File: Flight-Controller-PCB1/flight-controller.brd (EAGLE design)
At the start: 100 x 25.4 mm, 37 parts, among them J1 1981584-1, U1 MK20DX256VLH7, U2 TPS61200, U3 MINI54TAN, Y1 32.768KHz, Y2 16Mhz/8pF

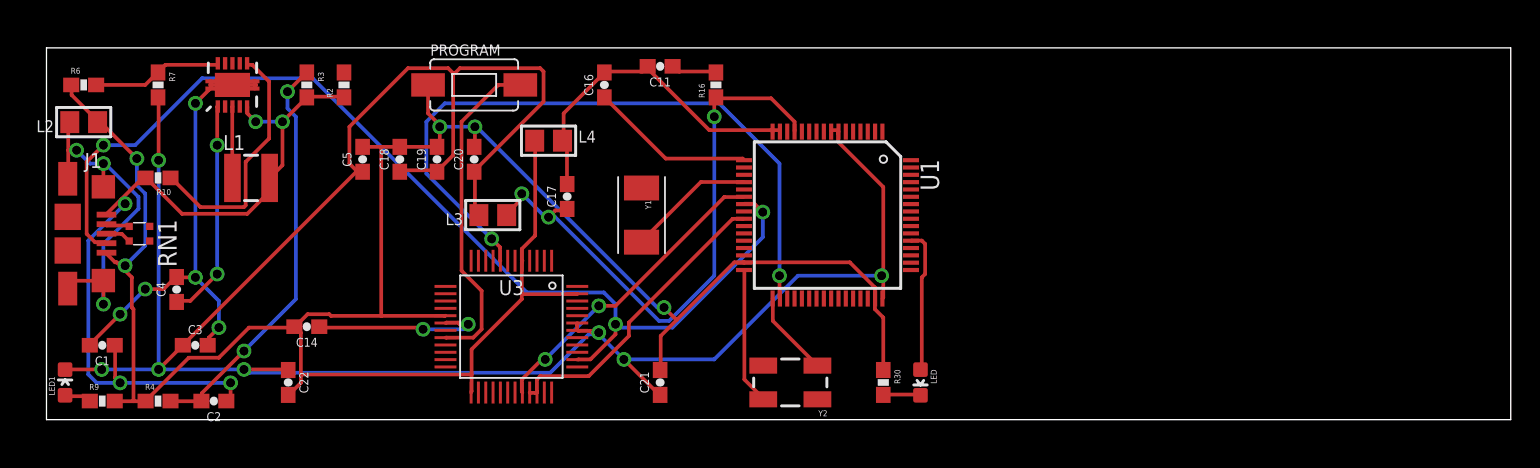
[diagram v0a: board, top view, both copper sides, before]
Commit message: update
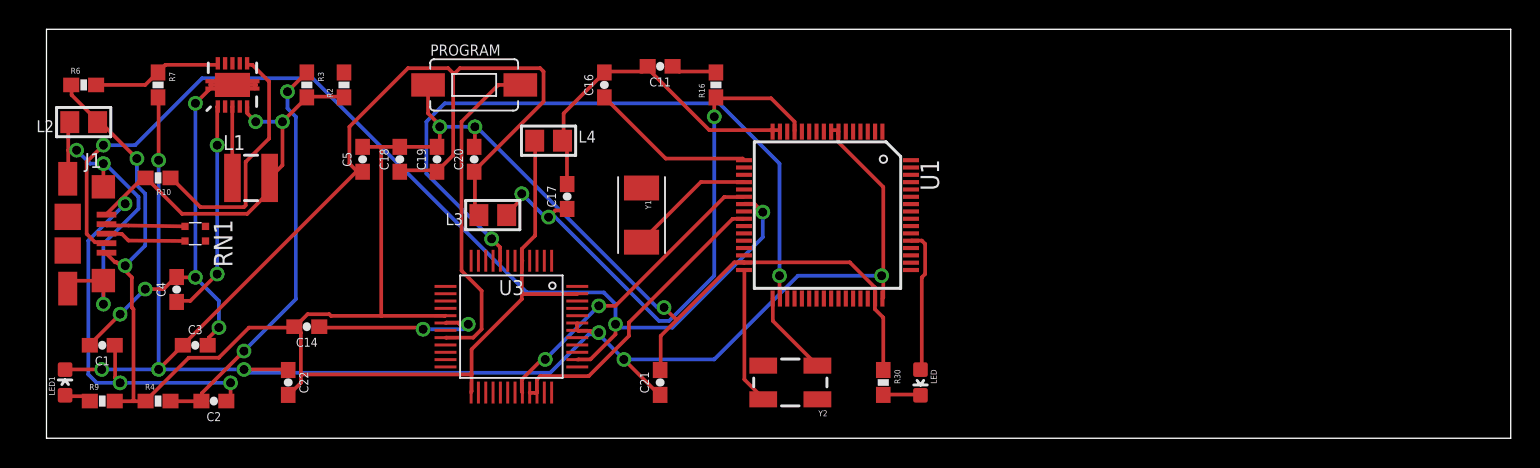
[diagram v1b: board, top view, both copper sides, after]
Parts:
- moved RN1 3.81 mm to (10.2, 12.7)
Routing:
- net USB_CON_P: track 1.75 -> 5.55 mm
- net USB_CON_N: track 1.66 -> 5.44 mm
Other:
- board size 100 x 25.4 mm -> 100 x 27.9 mm
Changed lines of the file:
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@@
 <board>
 <plain>
-<wire x1="0" y1="0" x2="100" y2="0" width="0" layer="20"/>
-<wire x1="100" y1="0" x2="100" y2="25.39" width="0" layer="20"/>
-<wire x1="100" y1="25.39" x2="0" y2="25.39" width="0" layer="20"/>
-<wire x1="0" y1="25.39" x2="0" y2="0" width="0" layer="20"/>
+<wire x1="0" y1="-1.27" x2="100" y2="-1.27" width="0" layer="20"/>
+<wire x1="100" y1="-1.27" x2="100" y2="26.66" width="0" layer="20"/>
+<wire x1="100" y1="26.66" x2="0" y2="26.66" width="0" layer="20"/>
+<wire x1="0" y1="26.66" x2="0" y2="-1.27" width="0" layer="20"/>
 </plain>
 <attributes>
@@
 <attribute name="MF" value="Panasonic" x="3.81" y="1.27" size="1.778" layer="27" display="off"/>
 </element>
-<element name="RN1" library="resistor-dil" package="EXB34V" value="33" x="6.35" y="12.7" rot="R270">
-<attribute name="MPN" value="EXB-34V330JV" x="6.35" y="12.7" size="1.778" layer="27" rot="R270" display="off"/>
-<attribute name="OC_NEWARK" value="unknown" x="6.35" y="12.7" size="1.778" layer="27" rot="R270" display="off"/>
-<attribute name="MF" value="Panasonic" x="6.35" y="12.7" size="1.778" layer="27" rot="R270" display="off"/>
-<attribute name="OC_FARNELL" value="unknown" x="6.35" y="12.7" size="1.778" layer="27" rot="R270" display="off"/>
+<element name="RN1" library="resistor-dil" package="EXB34V" value="33" x="10.16" y="12.7" rot="R270">
+<attribute name="MPN" value="EXB-34V330JV" x="10.16" y="12.7" size="1.778" layer="27" rot="R270" display="off"/>
+<attribute name="OC_NEWARK" value="unknown" x="10.16" y="12.7" size="1.778" layer="27" rot="R270" display="off"/>
+<attribute name="MF" value="Panasonic" x="10.16" y="12.7" size="1.778" layer="27" rot="R270" display="off"/>
+<attribute name="OC_FARNELL" value="unknown" x="10.16" y="12.7" size="1.778" layer="27" rot="R270" display="off"/>
 </element>
 <element name="U1" library="appfruits" package="MK20DX256VLH7" value="MK20DX256VLH7" x="53.34" y="13.97" rot="R270">
@@
 <contactref element="U1" pad="5"/>
 <contactref element="RN1" pad="3"/>
-<wire x1="7.05" y1="12.2" x2="55.09" y2="19.67" width="0" layer="19" extent="1-1"/>
+<wire x1="10.86" y1="12.2" x2="55.09" y2="19.67" width="0" layer="19" extent="1-1"/>
 </signal>
 <signal name="USB_D_N" class="1">
 <contactref element="RN1" pad="4"/>
 <contactref element="U1" pad="6"/>
-<wire x1="7.05" y1="13.2" x2="54.59" y2="19.67" width="0" layer="19" extent="1-1"/>
+<wire x1="10.86" y1="13.2" x2="54.59" y2="19.67" width="0" layer="19" extent="1-1"/>
 </signal>
 <signal name="ID">
@@
 <contactref element="RN1" pad="1"/>
 <wire x1="4.1148" y1="13.2588" x2="5.6007" y2="13.2588" width="0.254" layer="1"/>
-<wire x1="5.6007" y1="13.2588" x2="5.65" y2="13.2" width="0.254" layer="1"/>
+<wire x1="5.6007" y1="13.2588" x2="9.46" y2="13.2" width="0.254" layer="1"/>
 <wire x1="4.1148" y1="13.2588" x2="4.1" y2="13.35" width="0.254" layer="1"/>
 </signal>
@@
 <wire x1="5.1435" y1="12.6873" x2="5.6007" y2="12.2301" width="0.254" layer="1"/>
 <wire x1="4.1148" y1="12.6873" x2="5.1435" y2="12.6873" width="0.254" layer="1"/>
-<wire x1="5.6007" y1="12.2301" x2="5.65" y2="12.2" width="0.254" layer="1"/>
+<wire x1="5.6007" y1="12.2301" x2="9.46" y2="12.2" width="0.254" layer="1"/>
 <wire x1="4.1148" y1="12.6873" x2="4.1" y2="12.7" width="0.254" layer="1"/>
 </signal>

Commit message: started manually routing
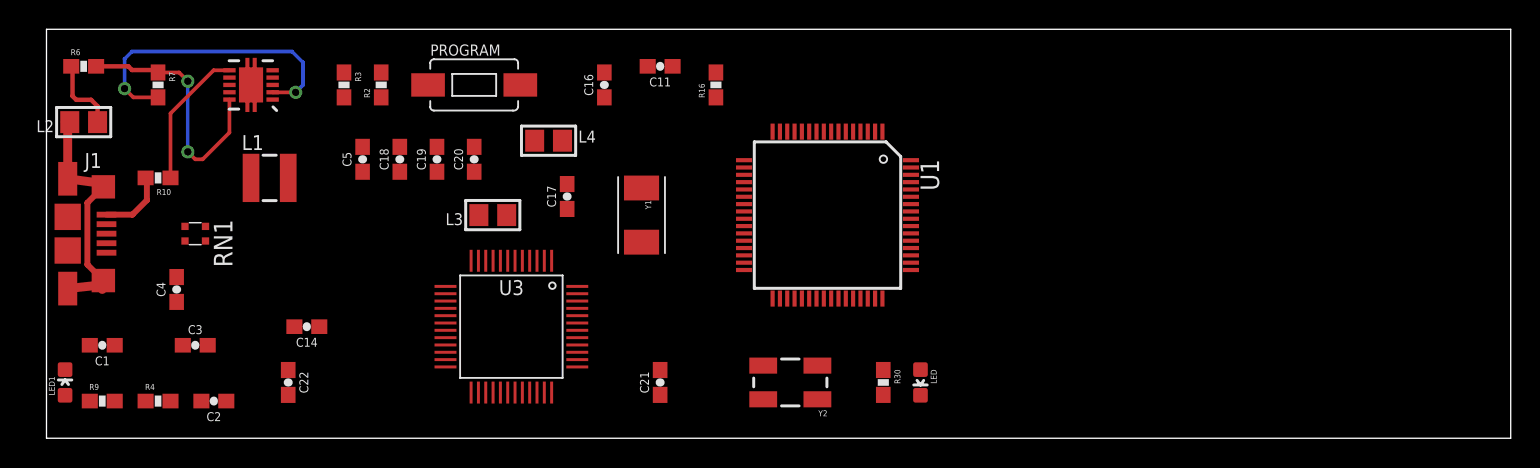
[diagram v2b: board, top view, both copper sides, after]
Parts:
- moved R2 2.54 mm to (22.9, 22.9)
- moved R3 2.54 mm to (20.3, 22.9)
- moved U2 1.27 mm to (14.0, 22.9), turned to 90 degrees
- moved L1 1.27 mm to (15.2, 16.5)
- moved R6 1.27 mm to (2.54, 24.1)
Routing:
- net GND: track 161.3 -> 5.15 mm, vias 5 -> 0
- net 3.3V: track 161.0 -> 21.1 mm, vias 7 -> 2
- net ID: track 72.7 -> 0.00 mm, vias 3 -> 0
- net VCC: track 54.1 -> 4.73 mm, vias 5 -> 0
- net RESET_B: track 47.2 -> 0.00 mm, vias 2 -> 0
- net VDDA: track 40.5 -> 0.00 mm, vias 3 -> 0
- net PGND: track 32.3 -> 0.00 mm, vias 5 -> 0
- net UVLO: track 28.0 -> 0.00 mm, vias 2 -> 0
- net VREFL: track 23.2 -> 0.00 mm
- net N$19: track 22.5 -> 0.00 mm
- net SWD_CLK: track 21.2 -> 0.00 mm, vias 2 -> 0
- net SWD_DIO: track 20.6 -> 0.00 mm
- net VAUX: track 15.1 -> 0.00 mm, vias 2 -> 0
- net N$22: track 12.0 -> 0.00 mm, vias 2 -> 0
- net VREF_OUT: track 11.3 -> 0.00 mm
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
